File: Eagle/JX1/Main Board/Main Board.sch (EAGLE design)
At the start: 10 parts, among them U1 SN74HC595N, U2 SN74HC595N

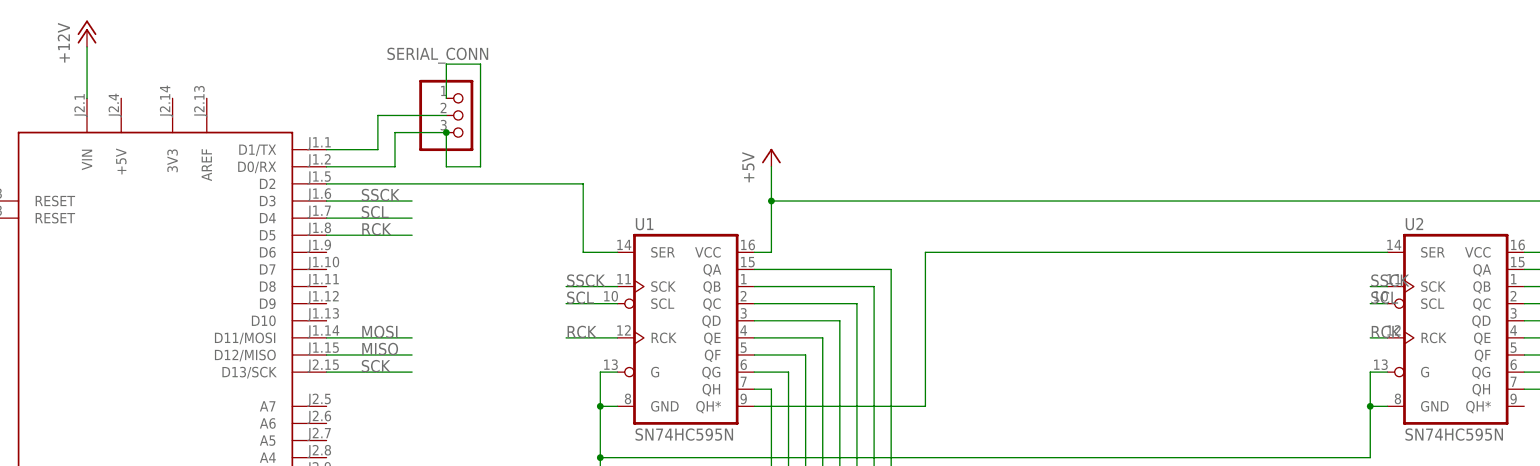
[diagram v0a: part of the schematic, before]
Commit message: Routed Main Board
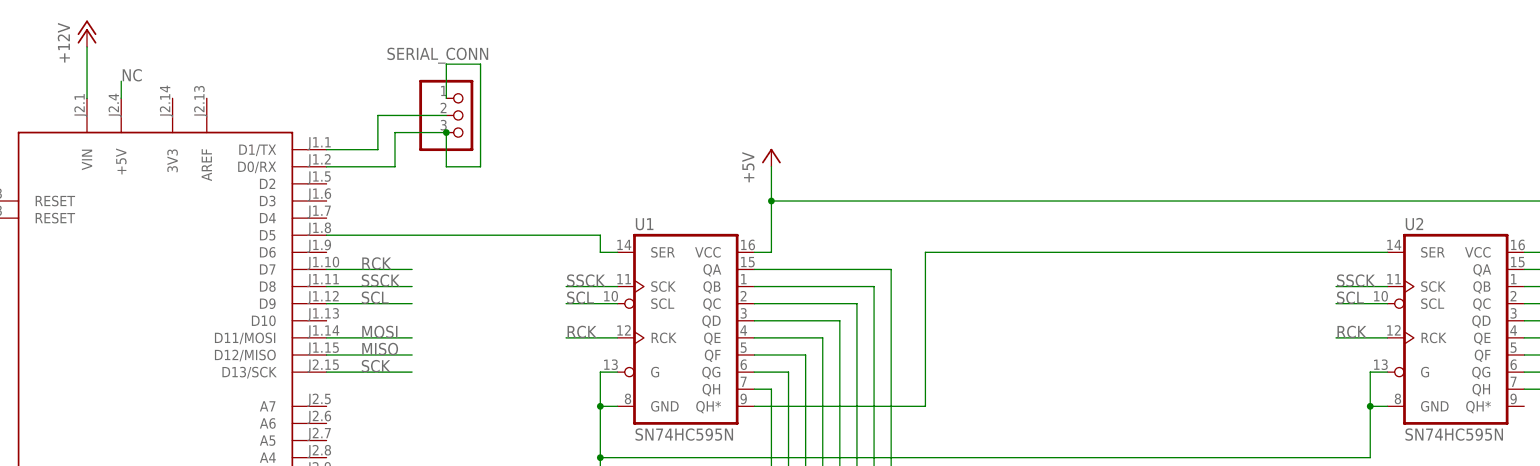
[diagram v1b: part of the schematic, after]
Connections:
- new net NC: MODUL1.+5V
- net N$22: now also MODUL1.D5; no longer MODUL1.D2
- net RCK: now also MODUL1.D7; no longer MODUL1.D5
- net SCL: now also MODUL1.D9; no longer MODUL1.D4
- net SSCK: now also MODUL1.D8; no longer MODUL1.D3
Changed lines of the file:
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@@
 </variantdefs>
 <classes>
-<class number="0" name="default" width="0" drill="0">
+<class number="0" name="default" width="0.254" drill="0">
 </class>
 <class number="1" name="Data" width="0.0254" drill="0">
@@
 <net name="N$22" class="1">
 <segment>
-<pinref part="MODUL1" gate="MODUL" pin="D2"/>
-<wire x1="73.66" y1="147.32" x2="111.76" y2="147.32" width="0.1524" layer="91"/>
-<wire x1="111.76" y1="147.32" x2="111.76" y2="137.16" width="0.1524" layer="91"/>
 <pinref part="U1" gate="U1" pin="SER"/>
-<wire x1="111.76" y1="137.16" x2="116.84" y2="137.16" width="0.1524" layer="91"/>
+<wire x1="114.3" y1="137.16" x2="116.84" y2="137.16" width="0.1524" layer="91"/>
+<pinref part="MODUL1" gate="MODUL" pin="D5"/>
+<wire x1="73.66" y1="139.7" x2="114.3" y2="139.7" width="0.1524" layer="91"/>
+<wire x1="114.3" y1="139.7" x2="114.3" y2="137.16" width="0.1524" layer="91"/>
 </segment>
 </net>
@@
 <segment>
 <pinref part="U2" gate="U1" pin="SCL"/>
-<wire x1="231.14" y1="129.54" x2="228.6" y2="129.54" width="0.1524" layer="91"/>
-<label x="228.6" y="129.54" size="1.778" layer="95"/>
+<wire x1="231.14" y1="129.54" x2="223.52" y2="129.54" width="0.1524" layer="91"/>
+<label x="223.52" y="129.54" size="1.778" layer="95"/>
 </segment>
 <segment>
@@
 </segment>
 <segment>
-<pinref part="MODUL1" gate="MODUL" pin="D4"/>
-<wire x1="86.36" y1="142.24" x2="73.66" y2="142.24" width="0.1524" layer="91"/>
-<label x="78.74" y="142.24" size="1.778" layer="95"/>
+<pinref part="MODUL1" gate="MODUL" pin="D9"/>
+<wire x1="73.66" y1="129.54" x2="86.36" y2="129.54" width="0.1524" layer="91"/>
+<label x="78.74" y="129.54" size="1.778" layer="95"/>
 </segment>
 </net>
@@
 <segment>
 <pinref part="U2" gate="U1" pin="RCK"/>
-<wire x1="231.14" y1="124.46" x2="228.6" y2="124.46" width="0.1524" layer="91"/>
-<label x="228.6" y="124.46" size="1.778" layer="95"/>
+<wire x1="231.14" y1="124.46" x2="223.52" y2="124.46" width="0.1524" layer="91"/>
+<label x="223.52" y="124.46" size="1.778" layer="95"/>
 </segment>
 <segment>
@@
 </segment>
 <segment>
-<pinref part="MODUL1" gate="MODUL" pin="D5"/>
-<wire x1="86.36" y1="139.7" x2="73.66" y2="139.7" width="0.1524" layer="91"/>
-<label x="78.74" y="139.7" size="1.778" layer="95"/>
+<pinref part="MODUL1" gate="MODUL" pin="D7"/>
+<wire x1="73.66" y1="134.62" x2="86.36" y2="134.62" width="0.1524" layer="91"/>
+<label x="78.74" y="134.62" size="1.778" layer="95"/>
 </segment>
 </net>
 <net name="SSCK" class="0">
-<segment>
-<pinref part="MODUL1" gate="MODUL" pin="D3"/>
-<wire x1="73.66" y1="144.78" x2="86.36" y2="144.78" width="0.1524" layer="91"/>
-<label x="78.74" y="144.78" size="1.778" layer="95"/>
-</segment>
 <segment>
 <pinref part="U1" gate="U1" pin="SCK"/>
@@
 <segment>
 <pinref part="U2" gate="U1" pin="SCK"/>
-<wire x1="231.14" y1="132.08" x2="228.6" y2="132.08" width="0.1524" layer="91"/>
-<label x="228.6" y="132.08" size="1.778" layer="95"/>
+<wire x1="231.14" y1="132.08" x2="223.52" y2="132.08" width="0.1524" layer="91"/>
+<label x="223.52" y="132.08" size="1.778" layer="95"/>
+</segment>
+<segment>
+<pinref part="MODUL1" gate="MODUL" pin="D8"/>
+<wire x1="73.66" y1="132.08" x2="86.36" y2="132.08" width="0.1524" layer="91"/>
+<label x="78.74" y="132.08" size="1.778" layer="95"/>
 </segment>
 </net>
@@
 </segment>
 </net>
-<net name="N$28" class="0">
+<net name="N$28" class="1">
 <segment>
 <pinref part="U1" gate="U1" pin="QH"/>
@@
 </segment>
 </net>
+<net name="NC" class="0">
+<segment>
+<pinref part="MODUL1" gate="MODUL" pin="+5V"/>
+<wire x1="43.18" y1="160.02" x2="43.18" y2="162.56" width="0.1524" layer="91"/>
+<label x="43.18" y="162.56" size="1.778" layer="95"/>
+</segment>
+</net>
